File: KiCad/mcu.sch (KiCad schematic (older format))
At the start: 36 parts, among them J13 SWD, J14 SDCARD, U3 STM32F407VGTx, Y1 16M

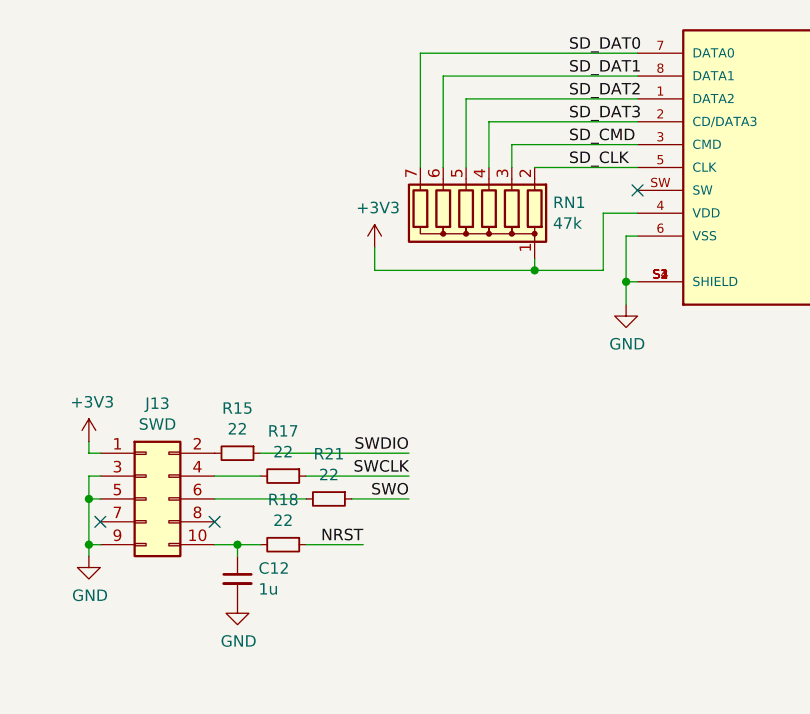
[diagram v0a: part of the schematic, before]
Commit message: FC PCB components layout
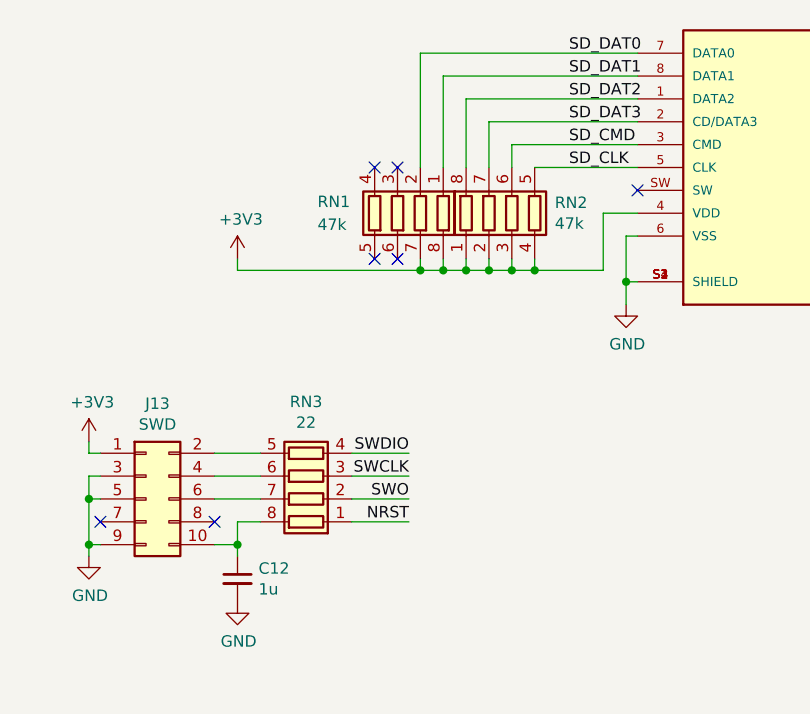
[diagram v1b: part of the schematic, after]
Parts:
- removed R15, R17, R18, R21: 22, Resistor_SMD:R_0603_1608Metric_Pad1.05x0.95mm_HandSolder, symbol Device:R_Small
- removed RN1: 47k, Resistor_THT:R_Array_SIP7, symbol Device:R_Network06
- added RN1, RN2: 47k, Resistor_SMD:R_Array_Concave_4x0603, symbol Device:R_Pack04
- added RN3: 22, Resistor_SMD:R_Array_Concave_4x0603, symbol Device:R_Pack04
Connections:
- net +3V3: now also RN1.7 (R2.2), RN1.8 (R1.2), RN2.1 (R1.1), RN2.2 (R2.1), RN2.3 (R3.1), RN2.4 (R4.1)
- net NRST: now also RN3.1 (R1.1)
- net SD_CLK: now also RN2.5 (R4.2)
- net SD_CMD: now also RN2.6 (R3.2)
- net SD_DAT0: now also RN1.2 (R2.1)
- net SD_DAT1: now also RN1.1 (R1.1)
- net SD_DAT2: now also RN2.8 (R1.2)
- net SD_DAT3: now also RN2.7 (R2.2)
- net SWCLK: now also RN3.3 (R3.1)
- net SWDIO: now also RN3.4 (R4.1)
- net SWO: now also RN3.2 (R2.1)
- net at C12.1, J13.10 (Pin_10): now also RN3.8 (R1.2)
- net at J13.2 (Pin_2): now also RN3.5 (R4.2)
- net at J13.4 (Pin_4): now also RN3.6 (R3.2)
- net at J13.6 (Pin_6): now also RN3.7 (R2.2)
- no-connect marks 51 -> 55
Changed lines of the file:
@@
 L power:+3V3 #PWR0140
 U 1 1 5FD77515
-P 6350 4550
-F 0 "#PWR0140" H 6350 4400 50  0001 C CNN
-F 1 "+3V3" H 6365 4723 50  0000 C CNN
-F 2 "" H 6350 4550 50  0001 C CNN
-F 3 "" H 6350 4550 50  0001 C CNN
-	1    6350 4550
+P 5750 4600
+F 0 "#PWR0140" H 5750 4450 50  0001 C CNN
+F 1 "+3V3" H 5765 4773 50  0000 C CNN
+F 2 "" H 5750 4600 50  0001 C CNN
+F 3 "" H 5750 4600 50  0001 C CNN
+	1    5750 4600
 	1    0    0    -1
 $EndComp
@@
 Text Label 6500 5450 2    50   ~ 0
 SWDIO
-$Comp
-L Device:R_Small R15
-U 1 1 5FFB97F1
-P 5750 5450
-F 0 "R15" V 5554 5450 50  0000 C CNN
-F 1 "22" V 5645 5450 50  0000 C CNN
-F 2 "Resistor_SMD:R_0603_1608Metric_Pad1.05x0.95mm_HandSolder" H 5750 5450 50  0001 C CNN
-F 3 "~" H 5750 5450 50  0001 C CNN
-	1    5750 5450
-	0    1    1    0
-$EndComp
-Wire Wire Line
-	5850 5450 6500 5450
+Wire Wire Line
+	6250 5450 6500 5450
 Text Label 6500 5550 2    50   ~ 0
 SWCLK
-$Comp
-L Device:R_Small R17
-U 1 1 5FFD99D3
-P 5950 5550
-F 0 "R17" V 5754 5550 50  0000 C CNN
-F 1 "22" V 5845 5550 50  0000 C CNN
-F 2 "Resistor_SMD:R_0603_1608Metric_Pad1.05x0.95mm_HandSolder" H 5950 5550 50  0001 C CNN
-F 3 "~" H 5950 5550 50  0001 C CNN
-	1    5950 5550
-	0    1    1    0
-$EndComp
-Wire Wire Line
-	6050 5550 6500 5550
+Wire Wire Line
+	6250 5550 6500 5550
 Text Label 6500 5650 2    50   ~ 0
 SWO
-$Comp
-L Device:R_Small R21
-U 1 1 5FFDECCF
-P 6150 5650
-F 0 "R21" V 5954 5650 50  0000 C CNN
-F 1 "22" V 6045 5650 50  0000 C CNN
-F 2 "Resistor_SMD:R_0603_1608Metric_Pad1.05x0.95mm_HandSolder" H 6150 5650 50  0001 C CNN
-F 3 "~" H 6150 5650 50  0001 C CNN
-	1    6150 5650
-	0    1    1    0
-$EndComp
 Wire Wire Line
 	6250 5650 6500 5650
-Wire Wire Line
-	5650 5550 5850 5550
-Wire Wire Line
-	5650 5650 6050 5650
 NoConn ~ 5650 5750
 Text Label 1400 1750 0    50   ~ 0
@@
 Wire Wire Line
 	1400 1750 1650 1750
-Text Label 6300 5850 2    50   ~ 0
+Text Label 6500 5750 2    50   ~ 0
 NRST
 $Comp
@@
 	1    0    0    -1
 $EndComp
-$Comp
-L Device:R_Small R18
-U 1 1 60044A42
-P 5950 5850
-F 0 "R18" V 5754 5850 50  0000 C CNN
-F 1 "22" V 5845 5850 50  0000 C CNN
-F 2 "Resistor_SMD:R_0603_1608Metric_Pad1.05x0.95mm_HandSolder" H 5950 5850 50  0001 C CNN
-F 3 "~" H 5950 5850 50  0001 C CNN
-	1    5950 5850
-	0    1    1    0
-$EndComp
 Wire Wire Line
 	5650 5850 5750 5850
@@
 Connection ~ 5750 5850
 Wire Wire Line
-	5750 5850 5850 5850
-Wire Wire Line
-	6050 5850 6300 5850
+	6250 5750 6500 5750
 $Comp
 L Device:Crystal_GND24_Small Y1
@@
 Text Label 3800 5950 2    50   ~ 0
 SD_DAT0
-$Comp
-L Device:R_Network06 RN1
-U 1 1 5FDD3900
-P 6750 4400
-F 0 "RN1" H 6370 4354 50  0000 R CNN
-F 1 "47k" H 6370 4445 50  0000 R CNN
-F 2 "Resistor_THT:R_Array_SIP7" V 7125 4400 50  0001 C CNN
-F 3 "http://www.vishay.com/docs/31509/csc.pdf" H 6750 4400 50  0001 C CNN
-	1    6750 4400
-	-1   0    0    1
-$EndComp
 Wire Wire Line
 	7500 4100 6950 4100
@@
 	6550 3700 6550 4200
 Wire Wire Line
-	6350 4550 6350 4650
-Wire Wire Line
-	6350 4650 7050 4650
+	5750 4600 5750 4650
 Wire Wire Line
 	7050 4650 7050 4600
@@
 	7350 4650 7050 4650
 Connection ~ 7050 4650
+$Comp
+L Device:R_Pack04 RN2
+U 1 1 5FE32852
+P 6950 4400
+F 0 "RN2" H 7138 4446 50  0000 L CNN
+F 1 "47k" H 7138 4355 50  0000 L CNN
+F 2 "Resistor_SMD:R_Array_Concave_4x0603" V 7225 4400 50  0001 C CNN
+F 3 "~" H 6950 4400 50  0001 C CNN
+	1    6950 4400
+	1    0    0    -1
+$EndComp
+Wire Wire Line
+	6950 4600 6950 4650
+Connection ~ 6950 4650
+Wire Wire Line
+	6950 4650 7050 4650
+Wire Wire Line
+	6850 4600 6850 4650
+Connection ~ 6850 4650
+Wire Wire Line
+	6850 4650 6950 4650
+Wire Wire Line
+	6750 4600 6750 4650
+Connection ~ 6750 4650
+Wire Wire Line
+	6750 4650 6850 4650
+Wire Wire Line
+	6650 4600 6650 4650
+Connection ~ 6650 4650
+Wire Wire Line
+	6650 4650 6750 4650
+Wire Wire Line
+	6550 4600 6550 4650
+Connection ~ 6550 4650
+Wire Wire Line
+	6550 4650 6650 4650
+$Comp
+L Device:R_Pack04 RN1
+U 1 1 5FE7310C
+P 6450 4400
+F 0 "RN1" H 6800 4350 50  0000 R CNN
+F 1 "47k" H 6800 4450 50  0000 R CNN
+F 2 "Resistor_SMD:R_Array_Concave_4x0603" V 6725 4400 50  0001 C CNN
+F 3 "~" H 6450 4400 50  0001 C CNN
+	1    6450 4400
+	-1   0    0    1
+$EndComp
+Wire Wire Line
+	5750 4650 6550 4650
+NoConn ~ 6350 4200
+NoConn ~ 6450 4200
+NoConn ~ 6350 4600
+NoConn ~ 6450 4600
+$Comp
+L Device:R_Pack04 RN3
+U 1 1 5FEA5572
+P 6050 5550
+F 0 "RN3" V 6375 5550 50  0000 C CNN
+F 1 "22" V 6284 5550 50  0000 C CNN
+F 2 "Resistor_SMD:R_Array_Concave_4x0603" V 6325 5550 50  0001 C CNN
+F 3 "~" H 6050 5550 50  0001 C CNN
+	1    6050 5550
+	0    -1   -1   0
+$EndComp
+Wire Wire Line
+	5650 5450 5850 5450
+Wire Wire Line
+	5650 5550 5850 5550
+Wire Wire Line
+	5850 5650 5650 5650
+Wire Wire Line
+	5750 5850 5750 5750
+Wire Wire Line
+	5750 5750 5850 5750
 $EndSCHEMATC
